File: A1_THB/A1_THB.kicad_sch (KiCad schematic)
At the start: 11 parts, among them J10 SFS, J11 Probe, J12 Hotend, J6 Thermister, J7 Conn_02x04_Odd_Even, J8 PCF, J9 EXF, Q1 NMOS

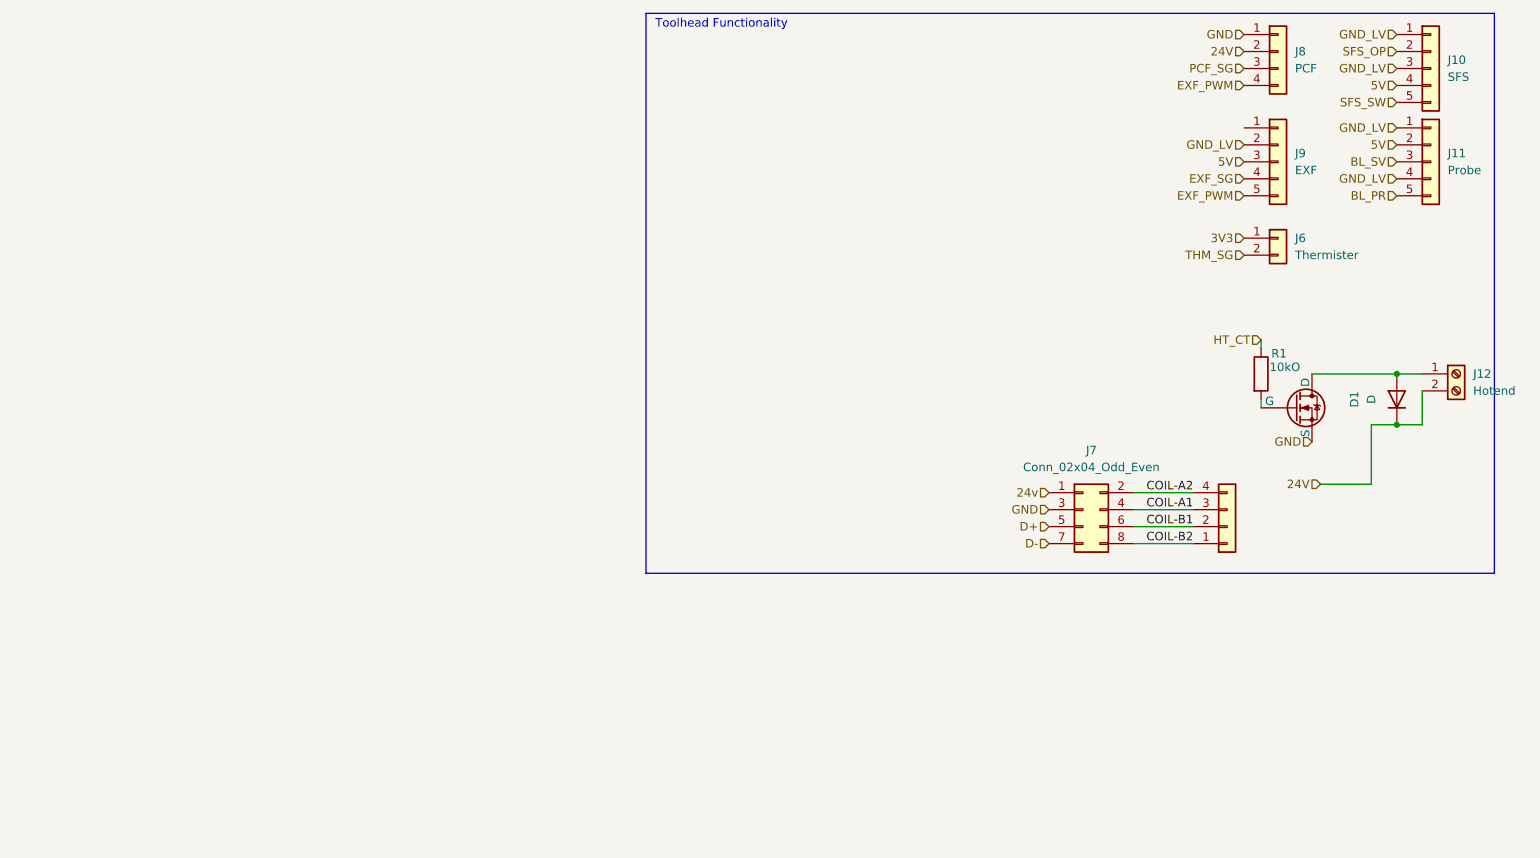
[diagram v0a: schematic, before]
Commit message: e
e
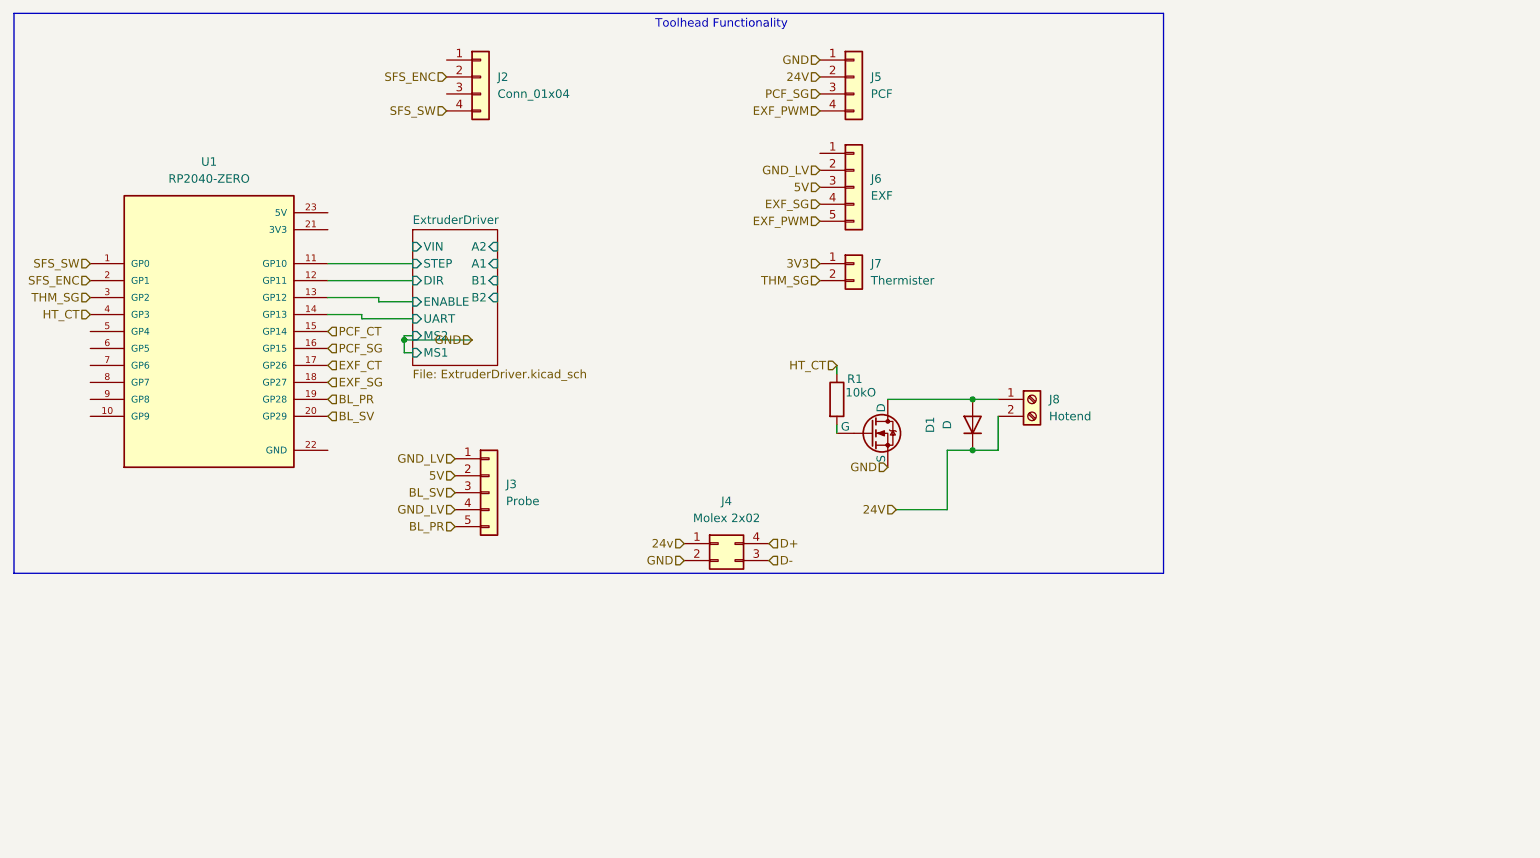
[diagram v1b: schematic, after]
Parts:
- removed ExtruderMotor1: Conn_01x04, Connector_JST:JST_XH_B4B-XH-AM_1x04_P2.50mm_Vertical, symbol Connector_Generic:Conn_01x04
- removed J10: SFS, Connector_PinHeader_2.54mm:PinHeader_1x05_P2.54mm_Vertical, symbol Connector_Generic:Conn_01x05
- removed J7: Conn_02x04_Odd_Even, Connector_Molex:Molex_Micro-Fit_3.0_43045-0818_2x04-1MP_P3.00mm_Vertical, symbol Connector_Generic:Conn_02x04_Odd_Even
- added J2: Conn_01x04, Connector_JST:JST_XH_B4B-XH-A_1x04_P2.50mm_Vertical, symbol Connector_Generic:Conn_01x04
- added J4: Molex 2x02, Connector_PinSocket_2.54mm:PinSocket_2x02_P2.54mm_Vertical, symbol Connector_Generic:Conn_02x02_Counter_Clockwise
- added U1: RP2040-ZERO, Libraries:RP2040-ZERO, symbol RP2040-ZERO:RP2040-ZERO
- D1: footprint (none) -> Diode_THT:D_5KPW_P12.70mm_Horizontal
- J8: renamed from J12; footprint Connector_JST:JST_XH_B2B-XH-AM_1x02_P2.50mm_Vertical -> OpenA1K:1x2 Terminal Block
- renumbered J11 to J3, J8 to J5, J9 to J6, J6 to J7
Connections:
- net 24v: now also J4.1 (Pin_1)
- net BL_PR: now also U1.19 (GP28)
- net BL_SV: now also U1.20 (GP29)
- net D+: now also J4.4 (Pin_4)
- net D-: now also J4.3 (Pin_3)
- net EXF_SG: now also U1.18 (GP27)
- net GND: now also J4.2 (Pin_2)
- net HT_CT: now also U1.4 (GP3)
- net PCF_SG: now also U1.16 (GP15)
- net SFS_SW: now also J2.4 (Pin_4), U1.1 (GP0)
- net THM_SG: now also U1.3 (GP2)
- new net EXF_CT: U1.17 (GP26)
- new net ExtruderDriver/DIR: U1.12 (GP11)
- new net ExtruderDriver/ENABLE: U1.13 (GP12)
- new net ExtruderDriver/STEP: U1.11 (GP10)
- new net ExtruderDriver/UART: U1.14 (GP13)
- new net PCF_CT: U1.15 (GP14)
- new net SFS_ENC: J2.2 (Pin_2), U1.2 (GP1)
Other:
- added sheet ExtruderDriver (ExtruderDriver.kicad_sch)
- moved on the sheet: D1, J3, J5, J6, J7, J8, R1

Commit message: e
e
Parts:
- J8: footprint OpenA1K:1x2 Terminal Block -> Libraries:CUI_TB004-508-05BE
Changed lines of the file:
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@@
 			)
 		)
-		(property "Footprint" "OpenA1K:1x2 Terminal Block"
+		(property "Footprint" "Libraries:CUI_TB004-508-05BE"
 			(at 171.45 120.65 0)
 			(effects

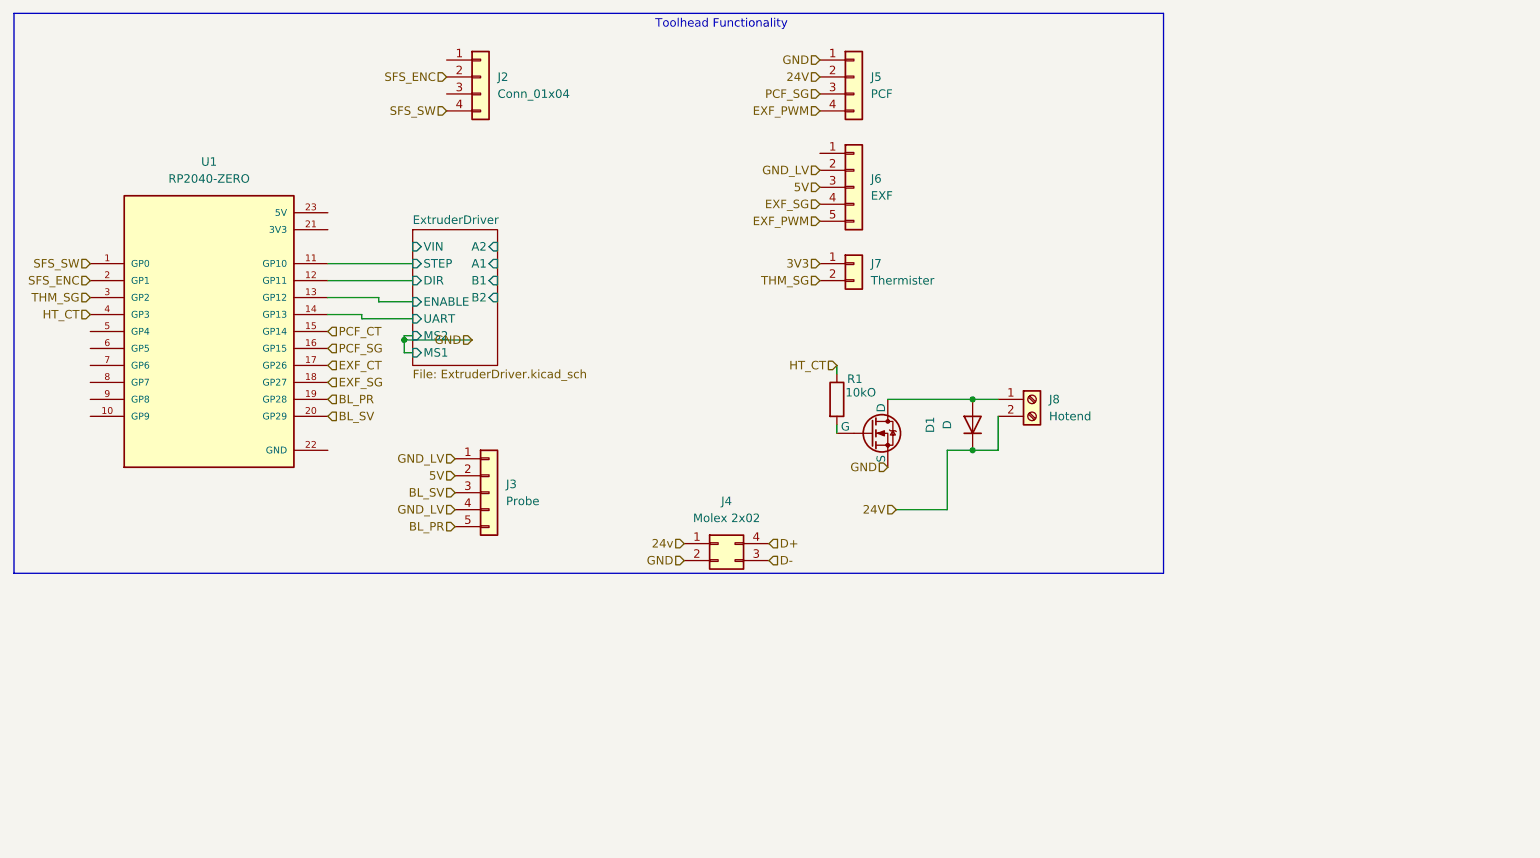
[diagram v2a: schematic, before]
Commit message: e
e
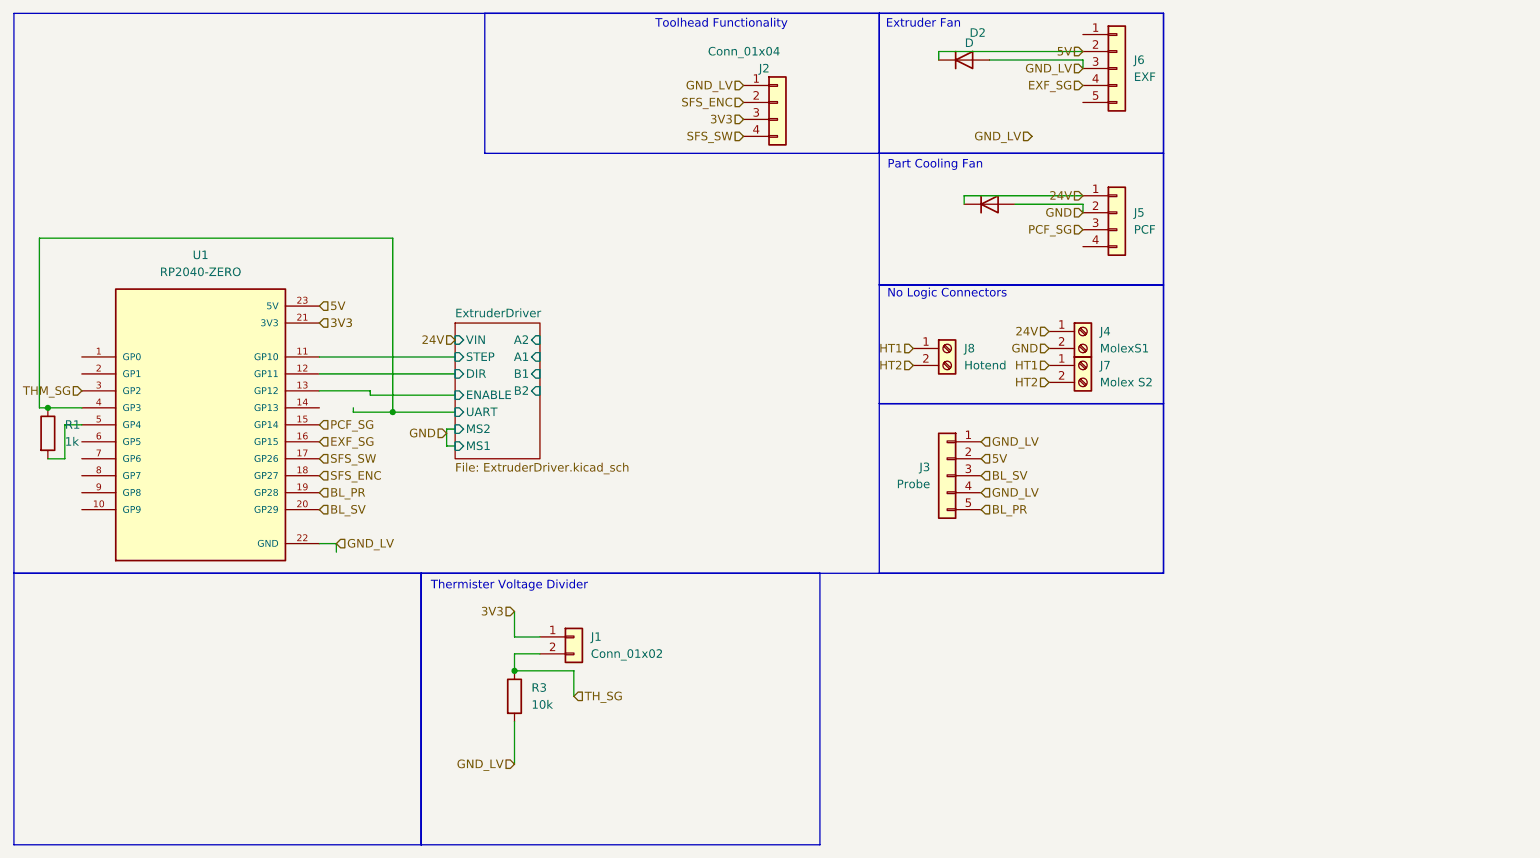
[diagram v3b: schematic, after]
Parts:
- removed D1: D, Diode_THT:D_5KPW_P12.70mm_Horizontal, symbol Device:D
- removed J4: Molex 2x02, Connector_PinSocket_2.54mm:PinSocket_2x02_P2.54mm_Vertical, symbol Connector_Generic:Conn_02x02_Counter_Clockwise
- removed J7: Thermister, Connector_JST:JST_XH_B2B-XH-AM_1x02_P2.50mm_Vertical, symbol Connector_Generic:Conn_01x02
- removed Q1: NMOS, symbol Simulation_SPICE:NMOS
- added D2, D3: D, A1_THB:DIOAD1036W78L470D235, symbol Device:D
- added J1: Conn_01x02, Connector_JST:JST_XH_B2B-XH-AM_1x02_P2.50mm_Vertical, symbol Connector_Generic:Conn_01x02
- added J4: MolexS1, OpenA1K:ScrewTerminal 7mm x 7mm, symbol Connector:Screw_Terminal_01x02
- added J7: Molex S2, OpenA1K:ScrewTerminal 7mm x 7mm, symbol Connector:Screw_Terminal_01x02
- added R3: 10k, symbol Device:R
- J8: footprint Libraries:CUI_TB004-508-05BE -> OpenA1K:ScrewTerminal 7mm x 7mm
- R1: value 10kO -> 1k
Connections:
- net EXF_CT is gone; now on net SFS_SW: U1.17 (GP26)
- net HT_CT is gone; now on net ExtruderDriver/UART: R1.1, U1.4 (GP3)
- net PCF_CT is gone; now on net PCF_SG: U1.15 (GP14)
- net 24V: now also J5.1 (Pin_1), D3.1 (K), J4.1 (Pin_1); no longer J5.2 (Pin_2), J8.2 (Pin_2)
- net 3V3: now also J2.3 (Pin_3), U1.21 (3V3), J1.1 (Pin_1)
- net 5V: now also J6.2 (Pin_2), U1.23 (5V), D2.1 (K); no longer J6.3 (Pin_3)
- net EXF_SG: now also U1.16 (GP15); no longer U1.18 (GP27)
- net ExtruderDriver/UART: no longer U1.14 (GP13)
- net GND: now also J5.2 (Pin_2), D3.2 (A), J4.2 (Pin_2); no longer J5.1 (Pin_1)
- net GND_LV: now also J2.1 (Pin_1), J6.3 (Pin_3), U1.22 (GND), D2.2 (A), R3.2; no longer J6.2 (Pin_2)
- net PCF_SG: no longer U1.16 (GP15)
- net SFS_ENC: now also U1.18 (GP27); no longer U1.2 (GP1)
- net SFS_SW: no longer U1.1 (GP0)
- net HT1: now reaches J8.1 (Pin_1)
- net HT1: now also J7.1 (Pin_1)
- net at R1.2: now also U1.5 (GP4)
- net EXF_PWM: no longer names the net of J5.4 (Pin_4)
- net EXF_PWM: no longer J6.5 (Pin_5)
- new net HT2: J7.2 (Pin_2), J8.2 (Pin_2)
- new net TH_SG: J1.2 (Pin_2), R3.1
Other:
- note added: "Extruder Fan"
- note added: "No Logic Connectors"
- note added: "Part Cooling Fan"
- note added: "Thermister Voltage Divider"
- moved on the sheet: J2, J3, J5, J6, U1
